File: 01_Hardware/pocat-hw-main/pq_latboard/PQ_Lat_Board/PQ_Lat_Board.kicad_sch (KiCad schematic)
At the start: 27 parts, among them IC1 TCN75AVOA713, J1 Conn_01x11_MountingPin, J2 Conn_Coaxial

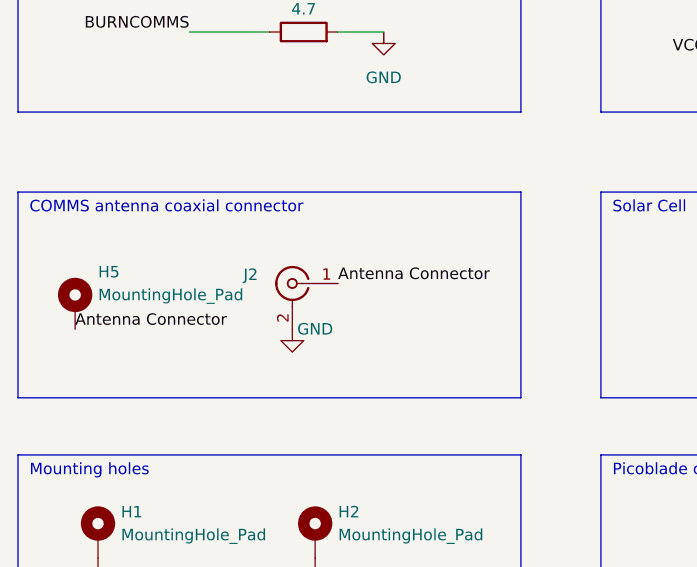
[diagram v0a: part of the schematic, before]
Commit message: Pcbs actualizados corregidos (son definitivos para mandarlos a fabricar con sus respectivos Gebers en una carpeta separada)
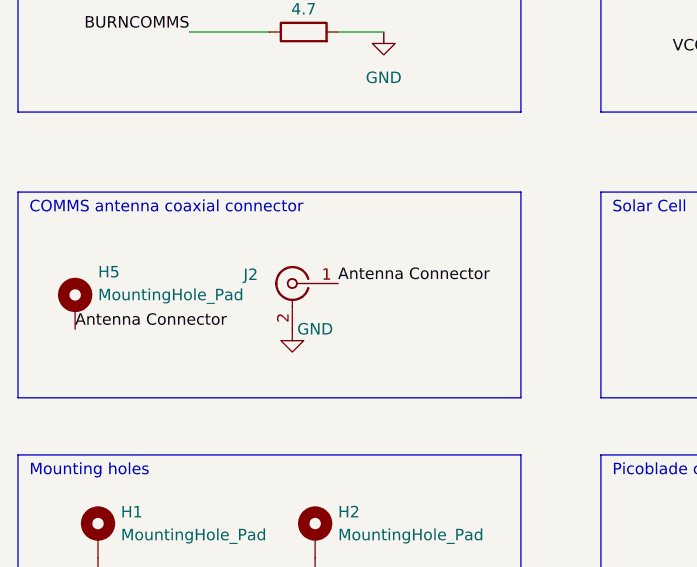
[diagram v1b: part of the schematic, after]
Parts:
- SC1: value ~ -> (none)
